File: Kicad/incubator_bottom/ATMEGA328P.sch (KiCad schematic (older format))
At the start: 5 parts, among them U3 ATmega328P-AU

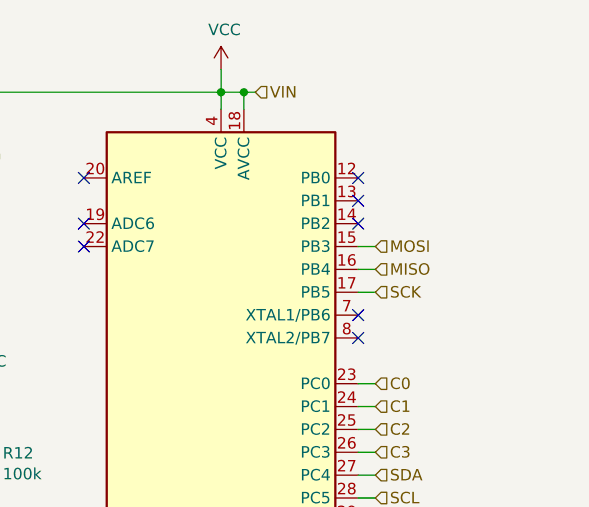
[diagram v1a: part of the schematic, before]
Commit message: feat: v1.0.1 of board
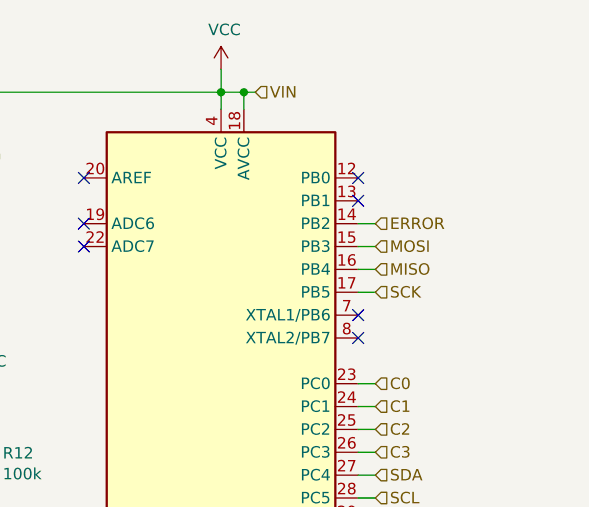
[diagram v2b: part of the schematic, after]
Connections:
- net ERROR: now reaches U3.14 (PB2)
- no-connect marks 8 -> 7
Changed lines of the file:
@@
 NoConn ~ 6775 2425
 NoConn ~ 6775 2525
-NoConn ~ 6775 2625
 NoConn ~ 6775 3025
 NoConn ~ 6775 3125
@@
 	0    1    1    0
 $EndComp
+Text HLabel 6850 2625 2    50   Input ~ 0
+ERROR
+Wire Wire Line
+	6775 2625 6850 2625
 $EndSCHEMATC
